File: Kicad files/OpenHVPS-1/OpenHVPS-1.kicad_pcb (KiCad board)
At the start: 2 copper layers, 77.5 x 20.5 mm, 71 parts, among them J1 Conn_01x03_Male, J2 Conn_01x03_Male, Q1 FQT7N10, Q2 BC846, Q3 MMDT3906, U1 74HC14, U2 MAX4162, U3 CD14538BM, U4 MAX6008AEUR+T

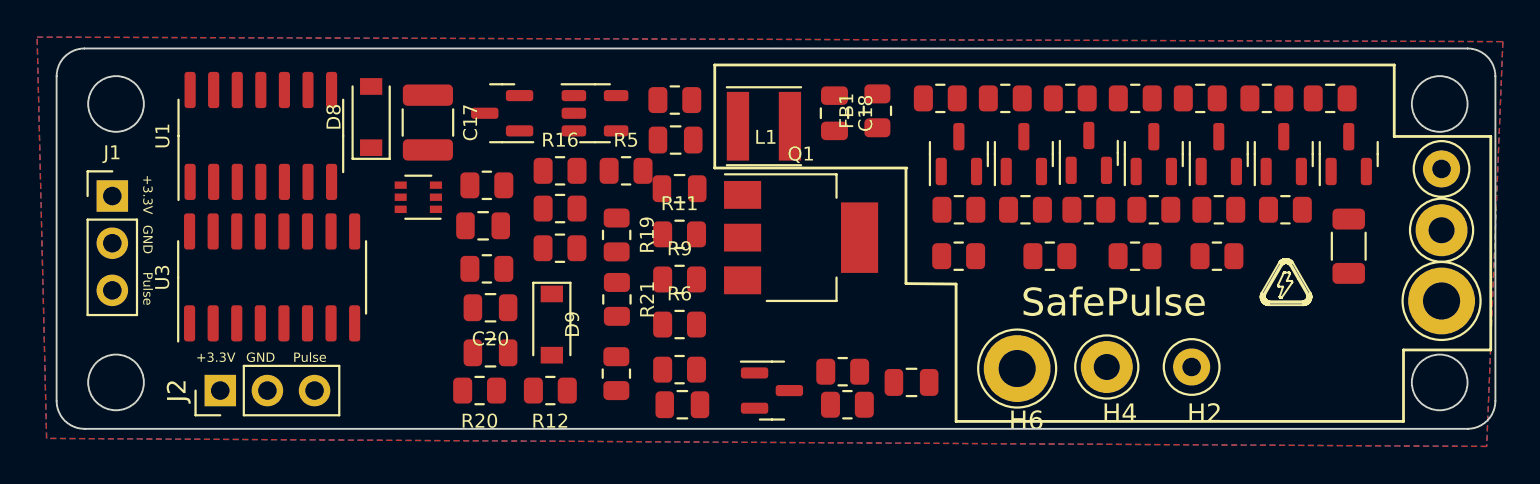
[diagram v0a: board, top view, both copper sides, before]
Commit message: cd \Users\allan\OneDrive\Documents\OpenHVPS  Please enter the commit message for your changes. Lines starting updated the long board design
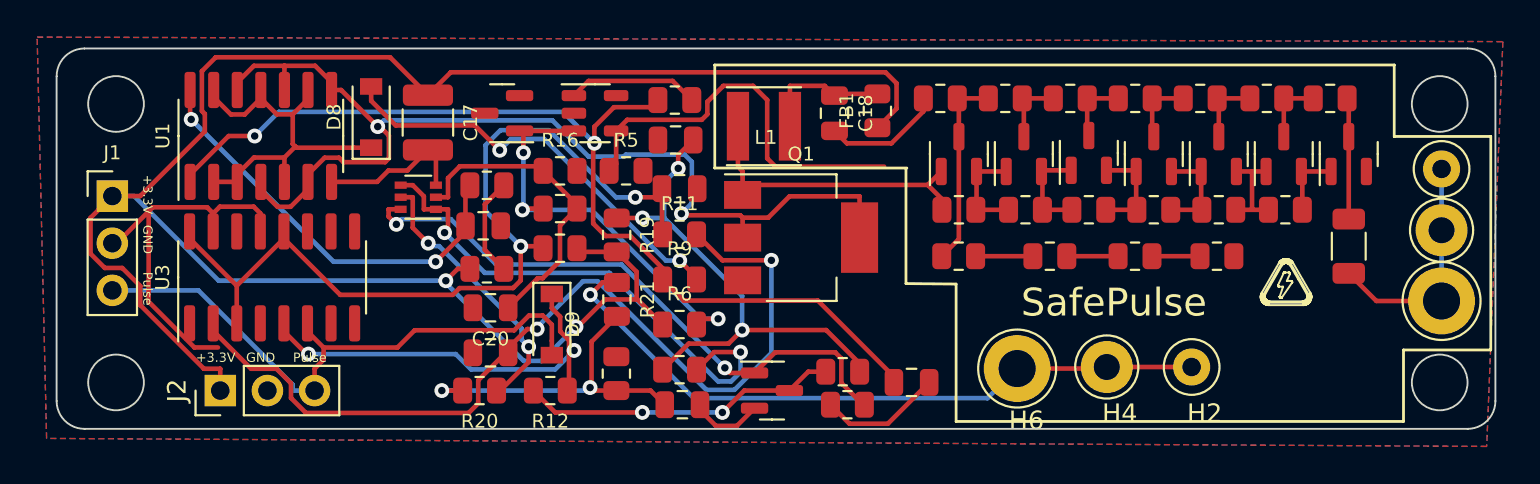
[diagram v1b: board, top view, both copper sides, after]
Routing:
- net +3V3: track 0.00 -> 108.9 mm, vias 0 -> 2
- net Net-(Q1-Pad2): track 0.00 -> 57.3 mm, vias 0 -> 2
- net Net-(C14-Pad1): track 0.00 -> 53.8 mm, vias 0 -> 2
- net Net-(C16-Pad1): track 0.00 -> 49.5 mm, vias 0 -> 2
- net Net-(C19-Pad1): track 0.00 -> 47.4 mm, vias 0 -> 2
- net GND: track 0.00 -> 45.9 mm
- net Net-(H2-Pad1): track 0.00 -> 37.1 mm, vias 0 -> 1
- net Net-(Q2-Pad1): track 0.00 -> 32.8 mm, vias 0 -> 2
- net Net-(D9-Pad2): track 0.00 -> 32.4 mm
- net Net-(Q3-Pad1): track 0.00 -> 28.1 mm, vias 0 -> 2
- net Net-(C21-Pad1): track 0.00 -> 27.9 mm, vias 0 -> 3
- net Net-(D9-Pad1): track 0.00 -> 23.2 mm, vias 0 -> 2
- net Net-(D8-Pad2): track 0.00 -> 22.8 mm, vias 0 -> 2
- net Net-(C15-Pad1): track 0.00 -> 22.8 mm, vias 0 -> 2
- net +2V5: track 0.00 -> 22.6 mm, vias 0 -> 3
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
